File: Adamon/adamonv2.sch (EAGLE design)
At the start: 15 parts, among them IC1 5V, U1 ATMEGA328P_PDIP_EZ, Y1 16 MHZ

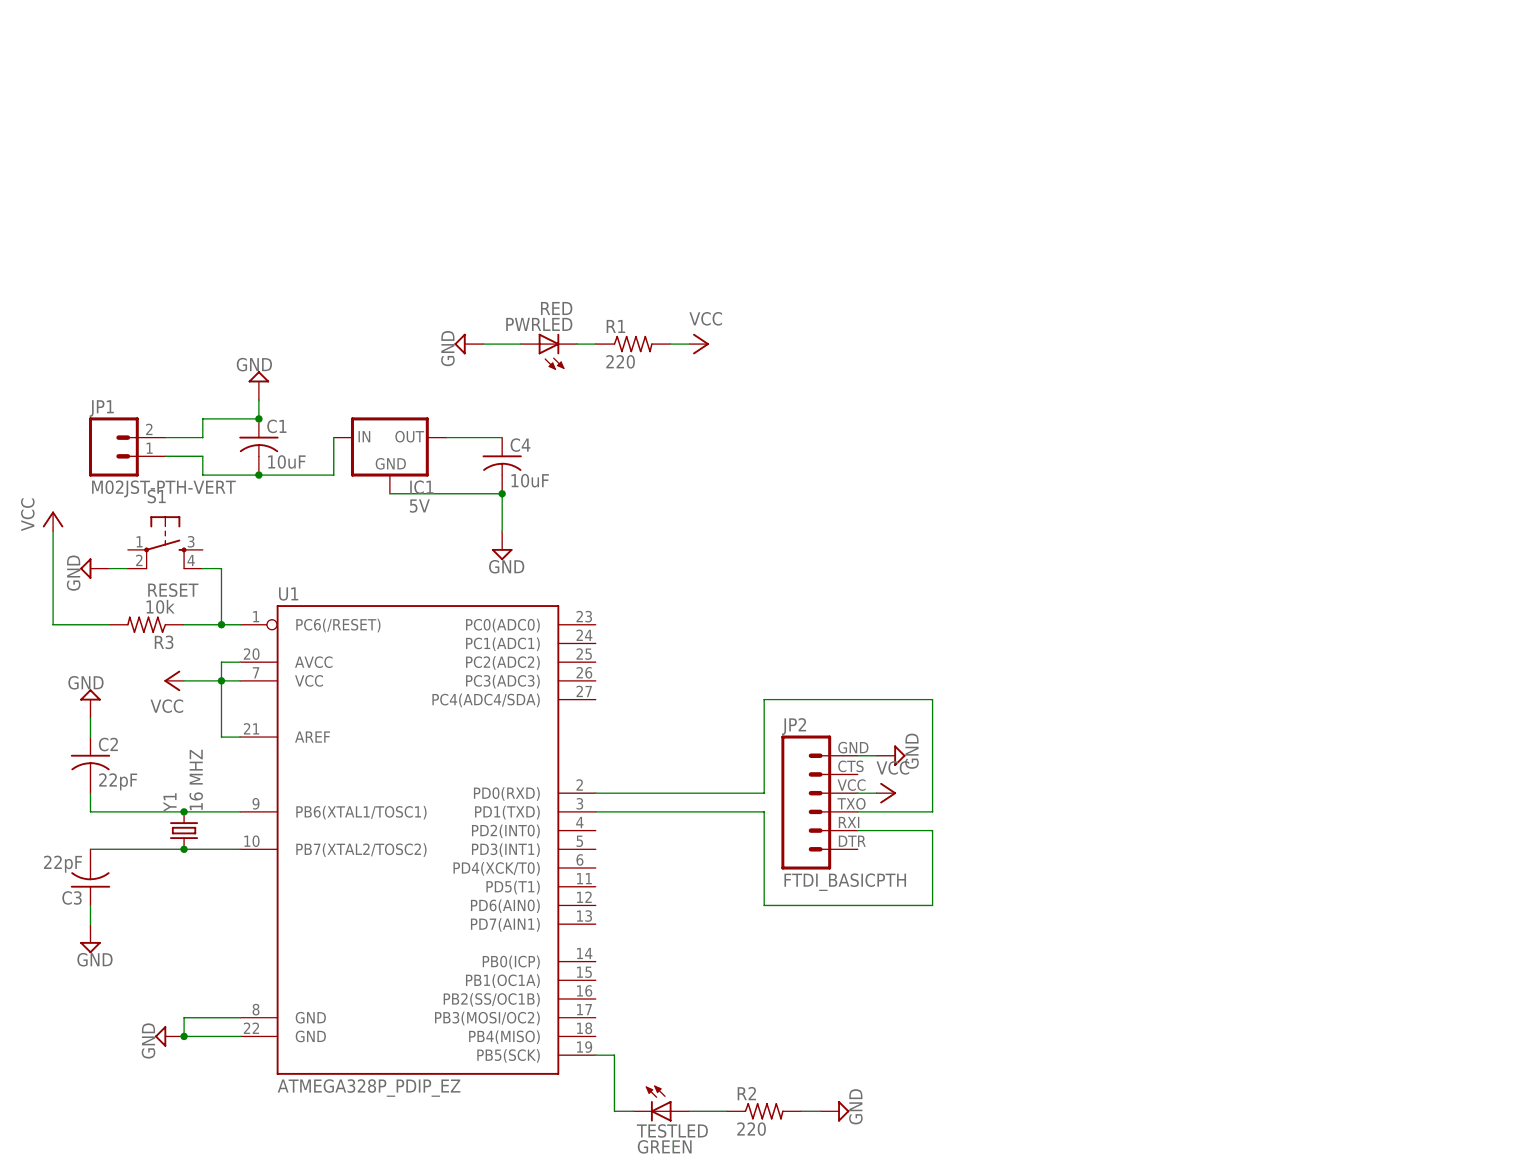
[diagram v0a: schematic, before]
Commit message: add stuff
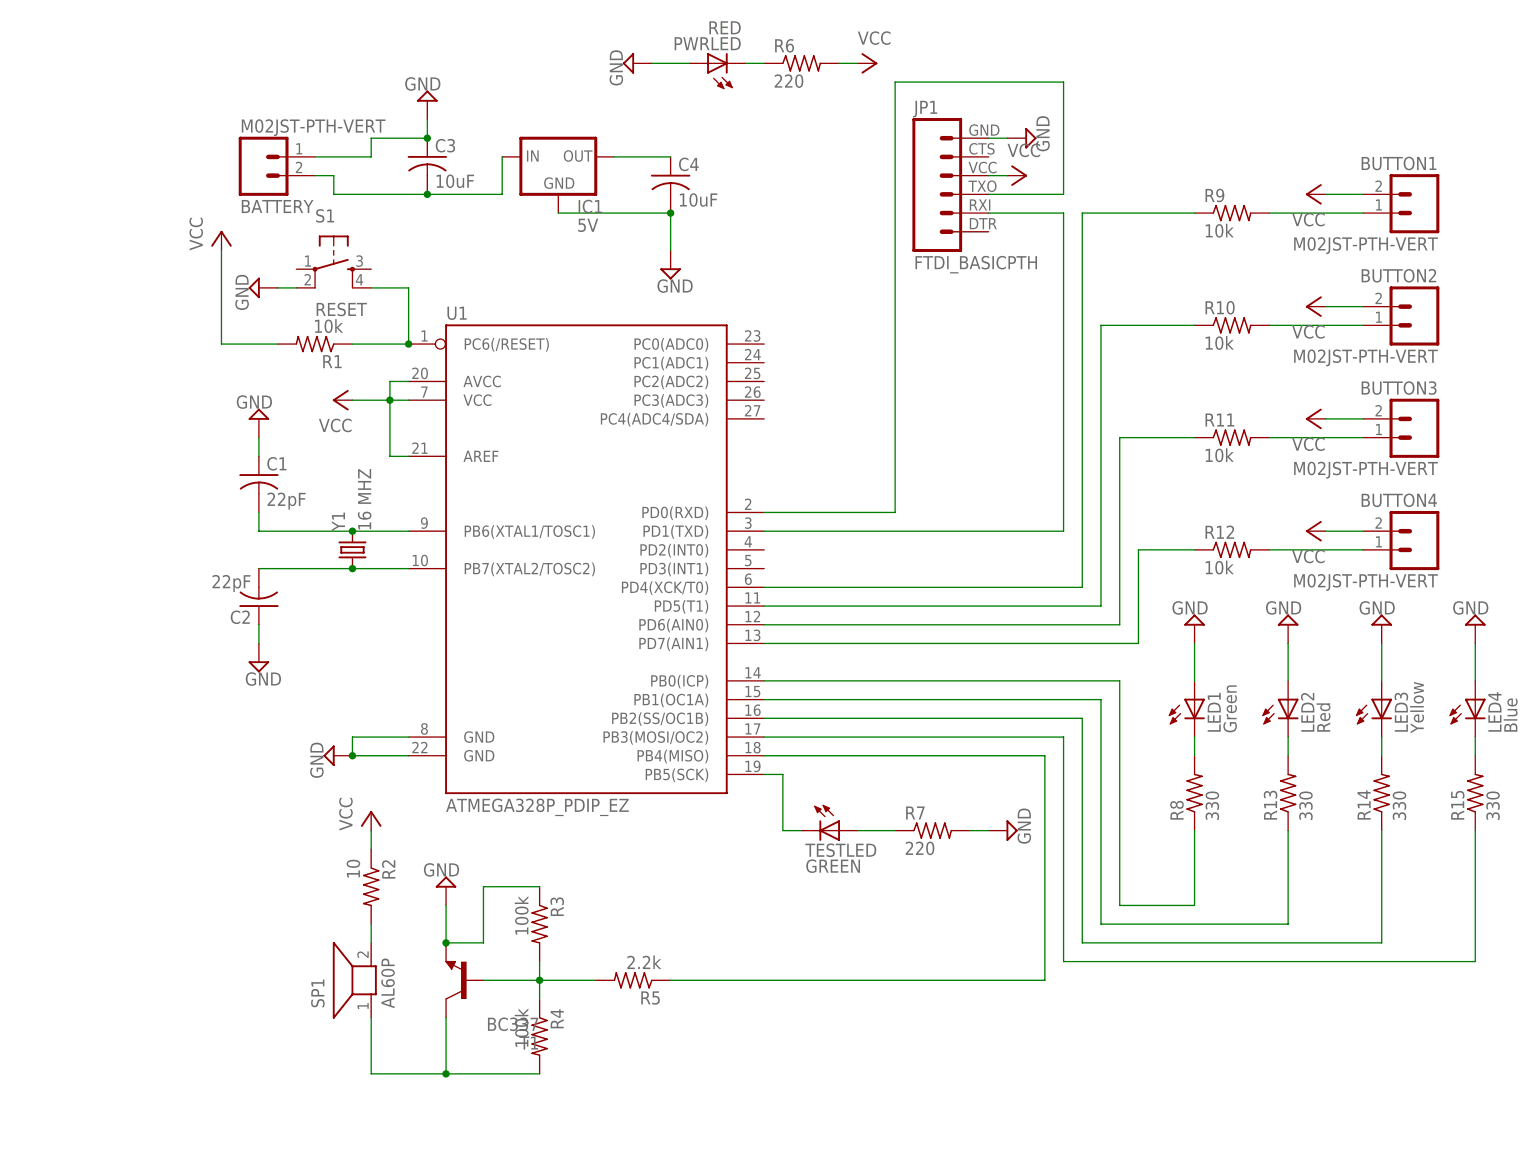
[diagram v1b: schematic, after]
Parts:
- removed JP2: FTDI_BASICPTH, SparkFun-Connectors:FTDI_BASICPTH
- added BATTERY, BUTTON1, BUTTON2, BUTTON3, BUTTON4: M02JST-PTH-VERT, SparkFun-Connectors:M02JST-PTH-VERT
- added LED1: Green, SparkFun-LED:LED5MM
- added LED2: Red, SparkFun-LED:LED5MM
- added LED3: Yellow, SparkFun-LED:LED5MM
- added LED4: Blue, SparkFun-LED:LED5MM
- added R10, R11, R12, R9: 10k, rcl:R-US_R0805
- added R13, R14, R15, R8: 330, rcl:R-US_R0805
- added R4: 100k, rcl:R-US_R0805
- added R5: 2.2k, rcl:R-US_R0805
- added R6, R7: 220, resistor:R-US_R0805
- added SP1: AL60P, buzzer:AL60P
- added T1: BC337, transistor:BC337
- C1: value 10uF -> 22pF
- C3: value 22pF -> 10uF
- JP1: value M02JST-PTH-VERT -> FTDI_BASICPTH; device SparkFun-Connectors:M02JST-PTH-VERT -> SparkFun-Connectors:FTDI_BASICPTH
- R1: value 220 -> 10k
- R2: value 220 -> 10; device resistor:R-US_R0805 -> rcl:R-US_R0805
- R3: value 10k -> 100k; device resistor:R-US_R0805 -> rcl:R-US_R0805
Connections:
- new net N$11: R15.1, U1.PB3(MOSI/OC2)
- new net N$12: R14.1, U1.PB2(SS/OC1B)
- new net N$13: R12.1, U1.PD7(AIN1)
- new net N$14: BUTTON1.1, R9.2
- new net N$15: R11.1, U1.PD6(AIN0)
- new net N$16: BUTTON2.1, R10.2
- new net N$17: R10.1, U1.PD5(T1)
- new net N$18: BUTTON3.1, R11.2
- new net N$19: R9.1, U1.PD4(XCK/T0)
- new net N$20: BUTTON4.1, R12.2
- new net N$24: R3.2, R4.1, R5.2, T1.B
- new net N$25: R4.2, SP1.1, T1.C
- new net N$26: R2.2, SP1.2
- new net N$31: R5.1, U1.PB4(MISO)
- new net N$32: LED4.C, R15.2
- new net N$33: LED3.C, R14.2
- new net N$34: R13.1, U1.PB1(OC1A)
- new net N$35: LED2.C, R13.2
- new net N$36: R8.1, U1.PB0(ICP)
- new net N$37: LED1.C, R8.2
- net GND: now also BATTERY.1, JP1.6, LED1.A, LED2.A, LED3.A, LED4.A, R3.1, R7.2, T1.E; no longer JP1.2, JP2.6, R2.2
- net N$1: now also C1.2; no longer C2.2
- net N$10: now also JP1.2; no longer JP2.2
- net N$2: now also BATTERY.2, C3.2; no longer C1.2, JP1.1
- net N$4: now also R6.1; no longer R1.1
- net N$5: now also R1.1; no longer R3.1
- net N$6: now also C2.2; no longer C3.2
- net N$8: now also R7.1; no longer R2.1
- net N$9: now also JP1.3; no longer JP2.3
- net VCC: now also BUTTON1.2, BUTTON2.2, BUTTON3.2, BUTTON4.2, JP1.4, R2.1, R6.2; no longer JP2.4, R3.2
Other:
- moved on the sheet: C1, C2, C3, C4, IC1, PWRLED, R1, R2, R3, S1, TESTLED, U1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
